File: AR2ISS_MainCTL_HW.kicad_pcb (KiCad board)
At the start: 4 copper layers, 200.7 x 111.8 mm, 332 parts, among them J1 Conn_01x06, J11 Conn_01x02, J12 Conn_01x02, J13 Conn_01x02, J14 Conn_01x02, J15 RJ45_LED, J16 Conn_01x02, J17 Conn_01x02, J18 Conn_02x17_Odd_Even, J19 Conn_02x17_Odd_Even, J2 Conn_01x06, J22 Conn_01x08, J23 Conn_01x08, J24 Conn_02x10_Odd_Even, J25 Conn_02x03_Odd_Even, J26 Conn_01x02, J27 Micro_SD_Card, J28 Conn_01x04, J3 Conn_01x02, J4 Conn_01x02, J5 Conn_01x08, J6 Conn_02x03_Odd_Even, J7 Conn_01x03, J8 DB9_Female, J9 Conn_01x02, K1 FINDER-34.51, K2 FINDER-34.51, K3 FINDER-34.51, K4 FINDER-34.51, Q1 BC846, Q2 BC846, Q3 BC846, Q4 BC846, Q7 PMN48XP, U1 MAX3232, U10 MCP23017_SO, U11 LME78_05-1.0, U12 L78033, U13 TSC101B, U14 TLE75602-ESH, U15 TLE75602-ESH, U16 MCP23017_SO, U17 LM358, U18 LM358, U19 SP3485EN-L/TR, U2 NUCLEO144-H745ZI, U3 SP3485EN-L/TR, U4 SP3485EN-L/TR, U5 SP3485EN-L/TR, U6 MCP2562-E-SN, U7 MCP23017_SO, U8 NTB0102DP, U9 74HC164

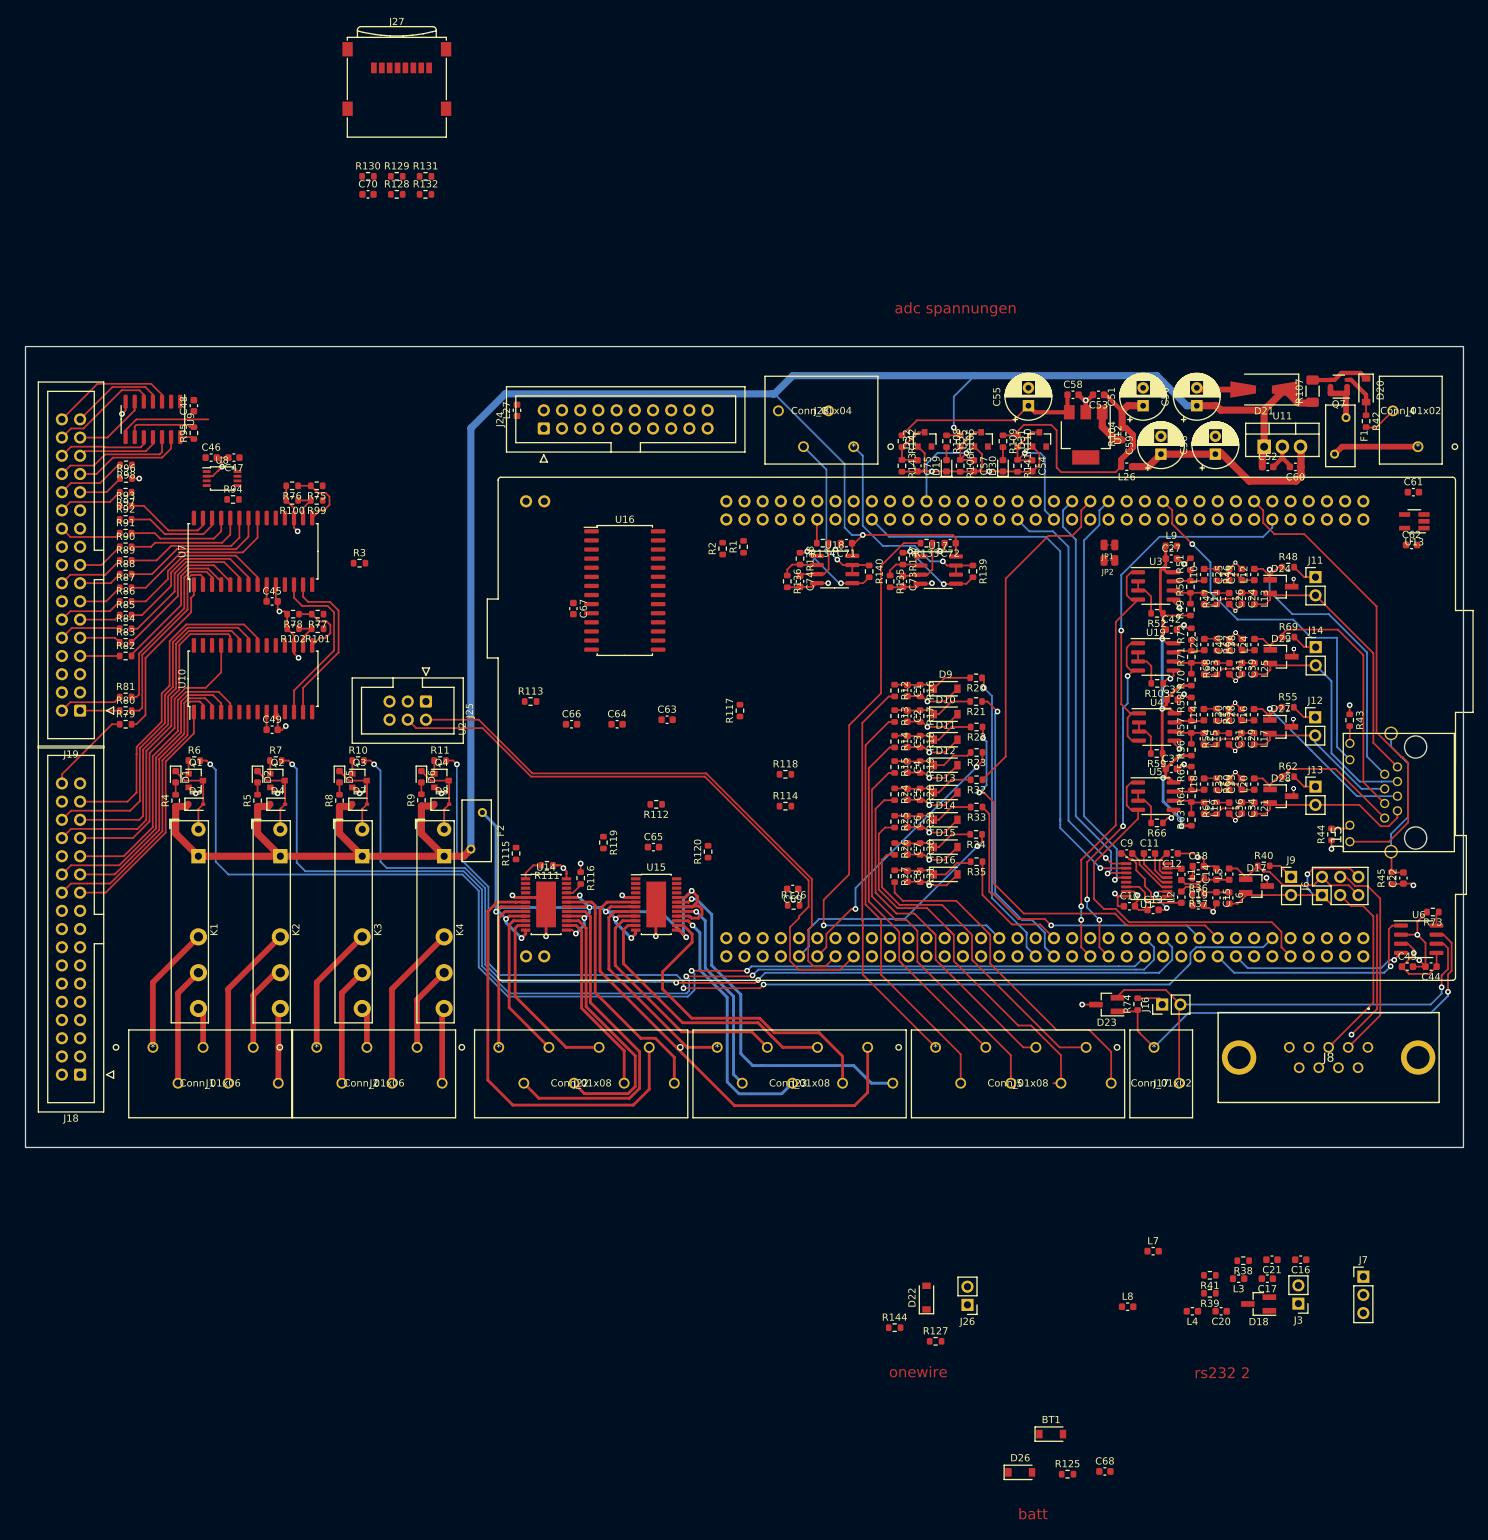
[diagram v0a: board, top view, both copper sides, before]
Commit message: ready for jlc
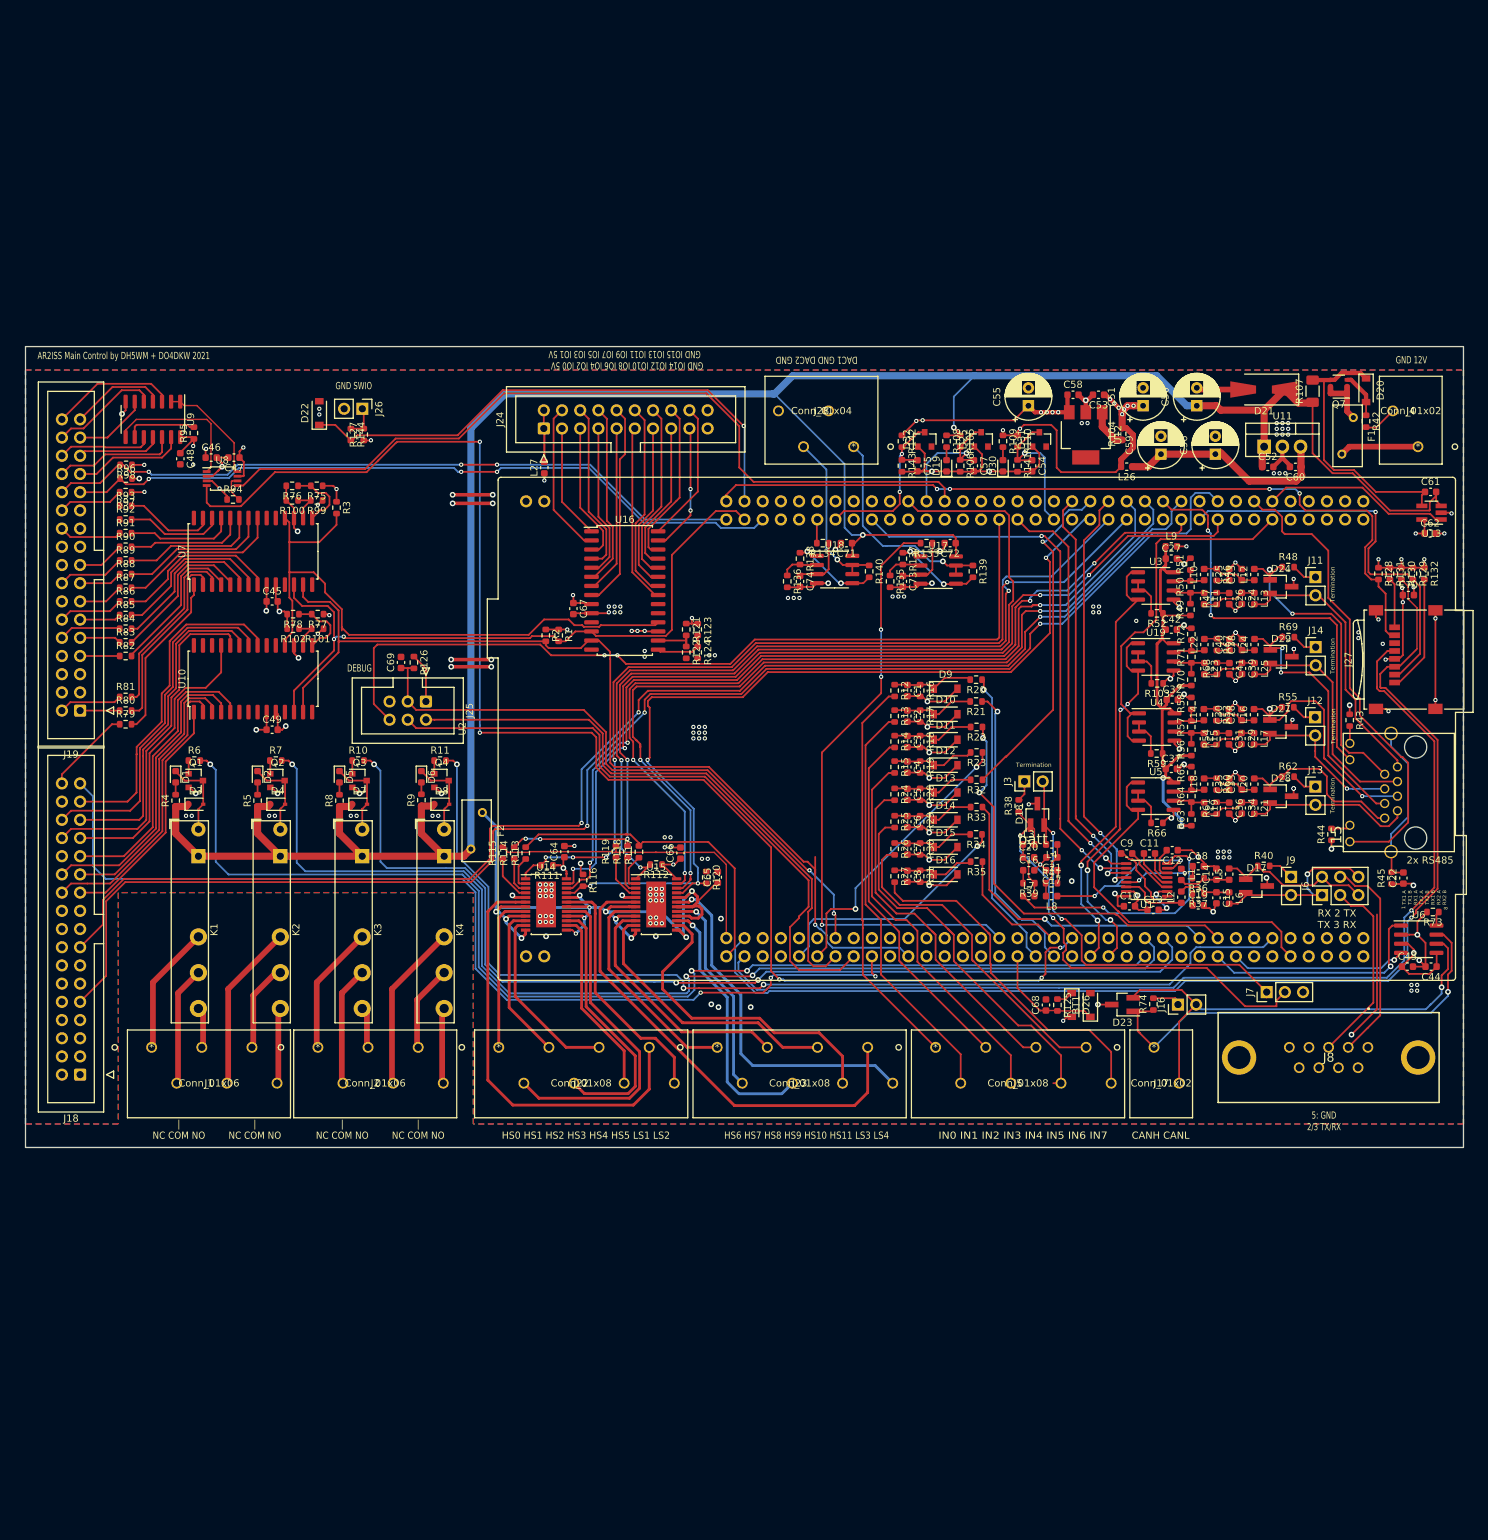
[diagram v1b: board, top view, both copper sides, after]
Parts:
- removed C63: 100nF, Capacitor_SMD:C_0603_1608Metric
- removed JP1, JP2: Jumper_NO_Small, AR2ISS:SOLDER_JUMPER
- added R121: 4.7k, Resistor_SMD:R_0603_1608Metric, F.Cu at (-372.8, -117.2)
- added R122: NB, Resistor_SMD:R_0603_1608Metric, F.Cu at (-372.8, -114.0)
- added R123: NB, Resistor_SMD:R_0603_1608Metric, F.Cu at (-371.2, -117.2)
- added R124: 0R, Resistor_SMD:R_0603_1608Metric, F.Cu at (-371.2, -114.0)
- moved J27 162.4 mm to (-272.4, -113.0), turned to 90 degrees
- moved C70 155.6 mm to (-272.0, -122.0)
- moved R130 154.5 mm to (-273.0, -125.0), turned to 270 degrees
- moved R129 152.2 mm to (-271.4, -125.0), turned to 270 degrees
- moved J26 150.9 mm to (-418.0, -147.9), turned to 270 degrees
- moved D22 149.7 mm to (-424.0, -147.3)
- moved R127 149.6 mm to (-417.8, -144.3), turned to 90 degrees
- moved R132 149.1 mm to (-269.8, -125.0), turned to 270 degrees
- moved R128 146.9 mm to (-276.2, -125.0), turned to 270 degrees
- moved R144 145.9 mm to (-419.6, -144.3), turned to 270 degrees
- moved R131 145.6 mm to (-274.6, -125.0), turned to 270 degrees
- moved J3 82.3 mm to (-325.6, -96.0), turned to 90 degrees
- moved D18 75.0 mm to (-323.8, -91.3), turned to 90 degrees
- moved R38 70.8 mm to (-326.4, -92.5), turned to 90 degrees
- moved C20 68.8 mm to (-325.0, -85.3), turned to 0 degrees
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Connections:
- U1 pad 13: /RS232/sheet608DD623/B_int -> /RS232/RS232Filter_1/A_int
- U1 pad 7: /RS232/RS232Filter_1/A_int -> /RS232/sheet608DD623/B_int
- U14 pad 22: /MESAOut/PWM_DOUT1 -> /Controller/PWM_DOUT1
- U14 pad 23: /MESAOut/PWM_DOUT0 -> /Controller/PWM_DOUT0
- U15 pad 22: /MESAOut/PWM_DOUT3 -> /Controller/PWM_DOUT3
- U15 pad 23: /MESAOut/PWM_DOUT2 -> /Controller/PWM_DOUT2
- U16 pad 17: /DOut/sheet60ADF1E9/A2 -> GND
- U2 pad 138: /Controller/CE -> Net-(U2-Pad138)
- U2 pad 139: /Controller/CD -> Net-(U2-Pad139)
- U2 pad 28: /Controller/ADC3V3 -> Net-(U2-Pad28)
- U2 pad 6: Net-(U2-Pad6) -> +5V
- U2 pad 73: Net-(U2-Pad73) -> /Controller/CD
- U2 pad 77: Net-(U2-Pad77) -> /Controller/CE
- U2 pad 85: /Controller/PWM_DOUT4 -> /Controller/ADC3V3
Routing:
- net /Controller/ENC_B: track 0.00 -> 206.5 mm, vias 0 -> 3
- net /Controller/DisplayCLK: track 0.00 -> 198.9 mm, vias 0 -> 5
- net /Controller/ENC_A: track 0.00 -> 191.7 mm, vias 0 -> 3
- net /SDCard/CMD: track 0.00 -> 164.9 mm, vias 0 -> 1
- net /SDCard/CLK: track 0.00 -> 148.3 mm, vias 0 -> 1
- net /Controller/Backlight: track 0.00 -> 140.6 mm, vias 0 -> 3
- net /Controller/PWM_DOUT0: track 0.00 -> 130.2 mm, vias 0 -> 4
- net /Controller/MOSI: track 0.00 -> 129.0 mm, vias 0 -> 4
- net /Controller/EN1: track 2.58 -> 131.3 mm, vias 0 -> 4
- net /Controller/PWM_DOUT1: track 0.00 -> 124.5 mm, vias 0 -> 4
- net /Controller/PWM_DOUT3: track 0.00 -> 121.0 mm, vias 0 -> 3
- net /Controller/#CS1: track 3.41 -> 123.5 mm, vias 0 -> 5
- net /Controller/PWM_DOUT2: track 0.00 -> 119.9 mm, vias 0 -> 3
- net /Controller/SWO: track 0.00 -> 118.6 mm, vias 0 -> 2
- net /Controller/#CS2: track 0.00 -> 115.4 mm, vias 0 -> 3
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- added copper zone on B.Cu, net +3V3
- added copper zone on In2.Cu, net +5V
- added copper zone on F.Cu, net GND
- removed copper zone on In2.Cu, net +3V3
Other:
- board text added: "1"
- board text added: "2x RS485"
- board text added: "5: GND 2/3 TX/RX"
- board text added: "8"
- board text added: "AR2ISS Main Control by DH5WM + DO4DKW 2021"
- board text added: "CANH CANL"
- board text added: "DAC1 GND DAC2 GND"
- board text added: "DEBUG"
- board text added: "GND 12V"
- board text added: "GND IO14 IO12 IO10 IO8 IO6 IO4 IO2 IO0 5V"
- board text added: "GND IO15 IO13 IO11 IO9 IO7 IO5 IO3 IO1 5V"
- board text added: "GND SWIO"
- board text added: "HS0 HS1 HS2 HS3 HS4 HS5 LS1 LS2"
- board text added: "HS6 HS7 HS8 HS9 HS10 HS11 LS3 LS4"
- board text added: "IN0 IN1 IN2 IN3 IN4 IN5 IN6 IN7"
- board text added: "RX 2 TX TX 3 RX"
- board text added: "TX1 A TX1 B RX1 A TX2 A TX2 B RX1 B RX2 A RX2 B"
- board text added: "Termination"
- board text added: "| NC COM NO"
- board text removed: "adc spannungen"
- board text removed: "onewire"
- board text removed: "rs232 2"

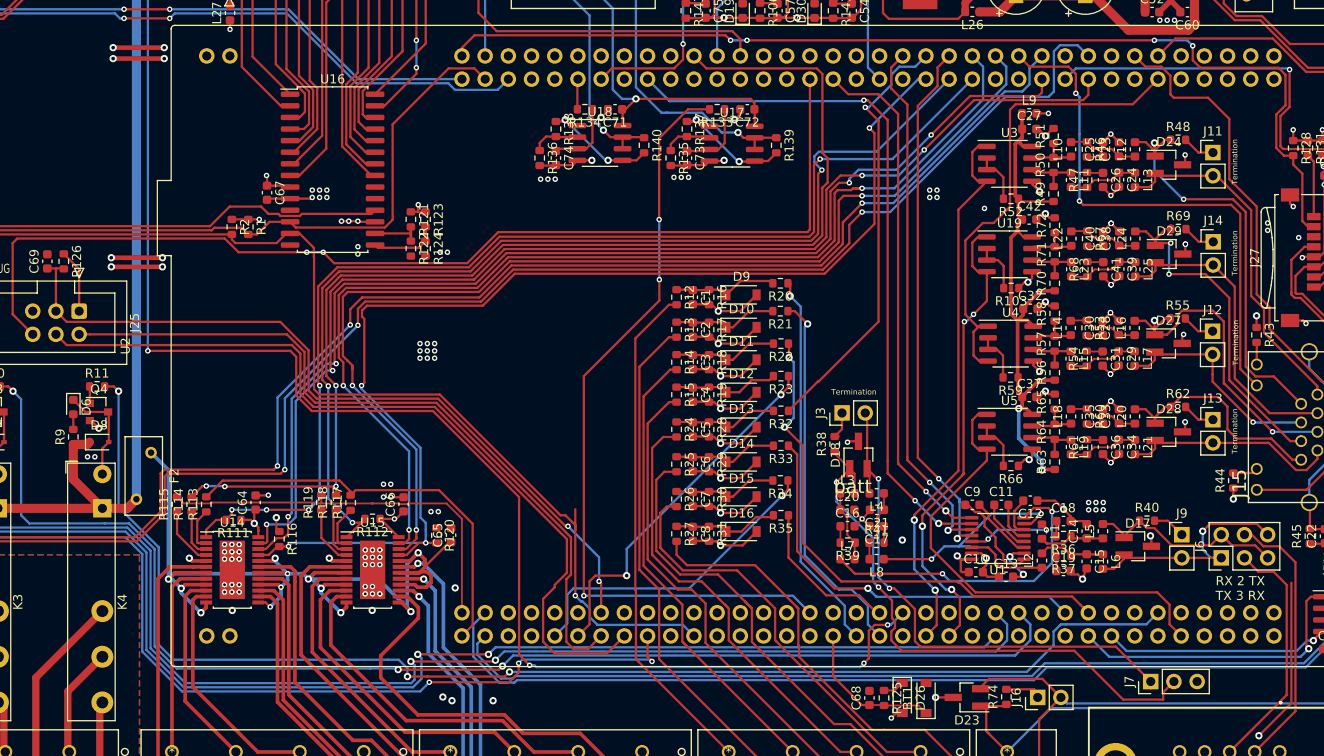
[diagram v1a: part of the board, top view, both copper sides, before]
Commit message: final routing
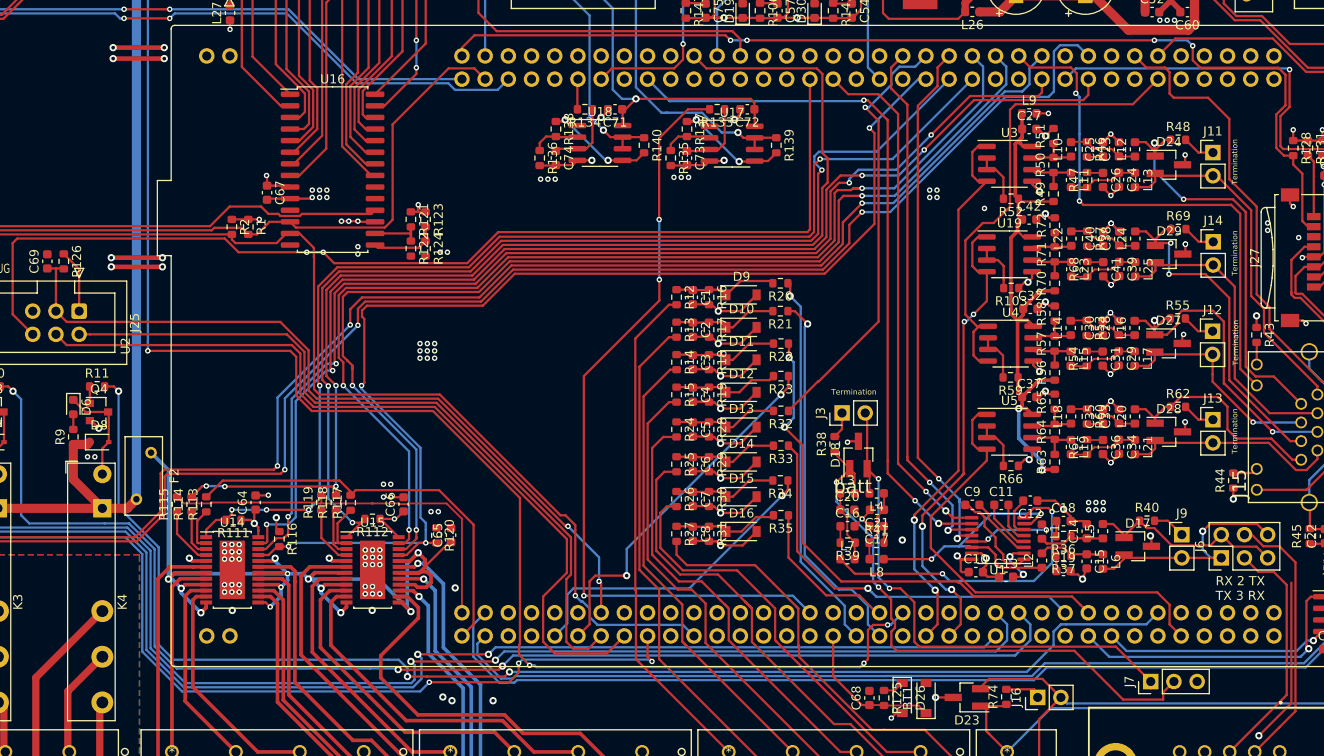
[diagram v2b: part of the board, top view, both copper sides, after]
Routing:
- net /Controller/SDA: track 139.0 -> 136.7 mm
- net +3V3: track 144.2 -> 142.8 mm
